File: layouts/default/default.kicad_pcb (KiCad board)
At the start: 2 copper layers, 13 parts

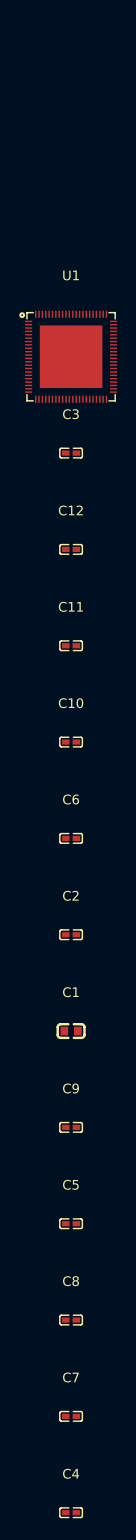
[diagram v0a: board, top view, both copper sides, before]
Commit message: initial build, migrating to V6
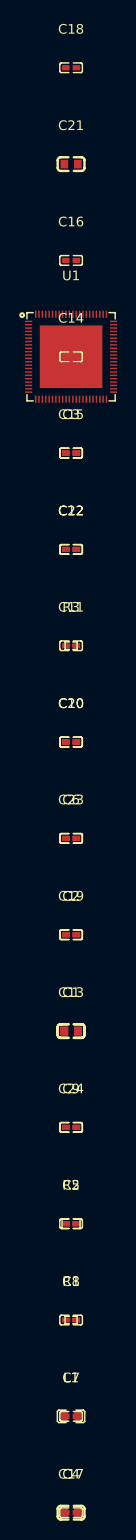
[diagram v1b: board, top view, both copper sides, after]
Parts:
- added C13: 100nF ±10% 50V X7R, atopile:C0603-bd72f6, F.Cu at (0.00, -50.0)
- added C14: 100nF ±10% 16V X7R, atopile:C0402-b3ef17, F.Cu at (0.00, -120.0)
- added C15: 100nF ±10% 16V X7R, atopile:C0402-b3ef17, F.Cu at (0.00, -110.0)
- added C16: 100nF ±10% 16V X7R, atopile:C0402-b3ef17, F.Cu at (0.00, -130.0)
- added C17: 100nF ±10% 50V X7R, atopile:C0603-bd72f6, F.Cu at (0.00, 0.00)
- added C18: 100nF ±10% 16V X7R, atopile:C0402-b3ef17, F.Cu at (0.00, -150.0)
- added C19: 100nF ±10% 16V X7R, atopile:C0402-b3ef17, F.Cu at (0.00, -60.0)
- added C20: 100nF ±10% 16V X7R, atopile:C0402-b3ef17, F.Cu at (0.00, -80.0)
- added C21: 100nF ±10% 50V X7R, atopile:C0603-bd72f6, F.Cu at (0.00, -140.0)
- added C22: 100nF ±10% 16V X7R, atopile:C0402-b3ef17, F.Cu at (0.00, -100.0)
- added C23: 100nF ±10% 16V X7R, atopile:C0402-b3ef17, F.Cu at (0.00, -70.0)
- added C24: 100nF ±10% 16V X7R, atopile:C0402-b3ef17, F.Cu at (0.00, -40.0)
- added L1: , atopile:L0603-9cac2b, F.Cu at (0.00, -10.0)
- added R1: 0Ω 50mW, atopile:R0201-27027e, F.Cu at (0.00, -20.0)
- added R2: 1kΩ ±1% 62.5mW, atopile:R0402-56259e, F.Cu at (0.00, -30.0)
- added R3: 0Ω 50mW, atopile:R0201-27027e, F.Cu at (0.00, -90.0)
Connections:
- net ETH_PHY_RXN renamed ETH_RN
- net ETH_PHY_RXP renamed ETH_RP
- net ETH_PHY_TXN renamed ETH_TN
- net ETH_PHY_TXP renamed ETH_TP
- net SDMMC0_DET_GPIO3_A1_u renamed SDMMC_DET
- C1 pad 1: C5-net-1 -> hv-2
- C1 pad 2: C5-net -> gnd
- C10 pad 1: C20-net -> hv-2
- C10 pad 2: C20-net-1 -> gnd
- C11 pad 1: C21-net-1 -> hv-2
- C11 pad 2: C21-net -> gnd
- C12 pad 1: C22-net -> hv-2
- C12 pad 2: C22-net-1 -> gnd
- C2 pad 1: C6-net -> hv-2
- C2 pad 2: C6-net-1 -> gnd
- C3 pad 1: C7-net-1 -> hv-2
- C3 pad 2: C7-net -> gnd
- C4 pad 1: C14-net -> hv-2
- C4 pad 2: C14-net-1 -> gnd
- C5 pad 1: C15-net -> hv-2
- C5 pad 2: C15-net-1 -> gnd
- C6 pad 1: C16-net -> hv-2
- C6 pad 2: C16-net-1 -> gnd
- C7 pad 1: C17-net -> hv-2
- C7 pad 2: C17-net-1 -> gnd
- C8 pad 1: C18-net-1 -> hv-2
- C8 pad 2: C18-net -> gnd
- C9 pad 1: C19-net -> hv-2
- C9 pad 2: C19-net-1 -> gnd
- U1 pad 11: SDMMC0_CLK_UART5_RTSN_M0_I2C0_SCL_M2_PWM10_M0_GPIO3_A4_d -> SDMMC_CLK_FL
- U1 pad 20: USB_AVDD3V3 -> hv-3
- U1 pad 34: DDR_VDDQ_1 -> VCC_DDR
- U1 pad 35: DDR_VDDQ_2 -> VCC_DDR
- U1 pad 36: DVDD -> hv-2
- U1 pad 38: DDR_PLL_AVDD1V8 -> hv-4
- U1 pad 39: DVDD -> hv-2
- U1 pad 40: DDR_VDDQ_3 -> VCC_DDR
- U1 pad 44: DVDD -> hv-2
- U1 pad 58: DVDD -> hv-2
- U1 pad 6: DVDD -> hv-2
- U1 pad 71: ETH_AVDD3V3 -> hv-3
- U1 pad 73: DVDD -> hv-2
- U1 pad 74: DVDD -> hv-2
- U1 pad 75: DVDD -> hv-2

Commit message: added flash and sd card
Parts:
- added R4: 1kΩ ±1% 62.5mW, atopile:R0402-56259e, F.Cu at (122.2, 51.2)
- added U2: , atopile:WSON-8_L6.0-W5.0-P1.27-BL-EP-5c84f1, F.Cu at (106.6, 164.0)
- added U3: , lib:TF-SMD_TF-01A, F.Cu at (132.2, 51.2)
- moved C1 204.0 mm to (106.6, 124.0)
- moved C10 204.0 mm to (106.6, 94.0)
- moved C11 204.0 mm to (106.6, 84.0)
- moved C12 204.0 mm to (106.6, 74.0)
- moved C13 204.0 mm to (106.6, 124.0)
- moved C14 204.0 mm to (106.6, 54.0)
- moved C15 204.0 mm to (106.6, 64.0)
- moved C16 204.0 mm to (106.6, 44.0)
- moved C18 204.0 mm to (106.6, 24.0)
- moved C19 204.0 mm to (106.6, 114.0)
- moved C2 204.0 mm to (106.6, 114.0)
- moved C20 204.0 mm to (106.6, 94.0)
- moved C21 204.0 mm to (106.6, 34.0)
- moved C22 204.0 mm to (106.6, 74.0)
- moved C23 204.0 mm to (106.6, 104.0)
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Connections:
- net C1-net renamed hv-5
- C1 pad 1: hv-2 -> hv
- C10 pad 1: hv-2 -> hv
- C11 pad 1: hv-2 -> hv
- C12 pad 1: hv-2 -> hv
- C13 pad 2: C1-net-1 -> gnd
- C14 pad 1: hv-3 -> hv-2
- C15 pad 1: hv-3 -> hv-2
- C17 pad 1: C8-net-1 -> C8-net
- C17 pad 2: C8-net -> C8-net-1
- C18 pad 1: C9-net -> C9-net-1
- C18 pad 2: C9-net-1 -> C9-net
- C2 pad 1: hv-2 -> hv
- C20 pad 1: C11-net-1 -> C11-net
- C20 pad 2: C11-net -> C11-net-1
- C21 pad 1: hv-1 -> hv-3
- C22 pad 1: hv-1 -> hv-3
- C3 pad 1: hv-2 -> hv
- C4 pad 1: hv-2 -> hv
- C5 pad 1: hv-2 -> hv
- C6 pad 1: hv-2 -> hv
- C7 pad 1: hv-2 -> hv
- C8 pad 1: hv-2 -> hv
- C9 pad 1: hv-2 -> hv
- L1 pad 2: hv-1 -> hv-3
- R2 pad 2: hv -> hv-1
- U1 pad 20: hv-3 -> hv-2
- U1 pad 36: hv-2 -> hv
- U1 pad 39: hv-2 -> hv
- U1 pad 44: hv-2 -> hv
- U1 pad 58: hv-2 -> hv
- U1 pad 6: hv-2 -> hv
- U1 pad 71: hv-3 -> hv-2
- U1 pad 73: hv-2 -> hv
- U1 pad 74: hv-2 -> hv
- U1 pad 75: hv-2 -> hv
